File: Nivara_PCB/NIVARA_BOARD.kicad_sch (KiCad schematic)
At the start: 3 parts, among them U18 ESP32-S3-WROOM-1

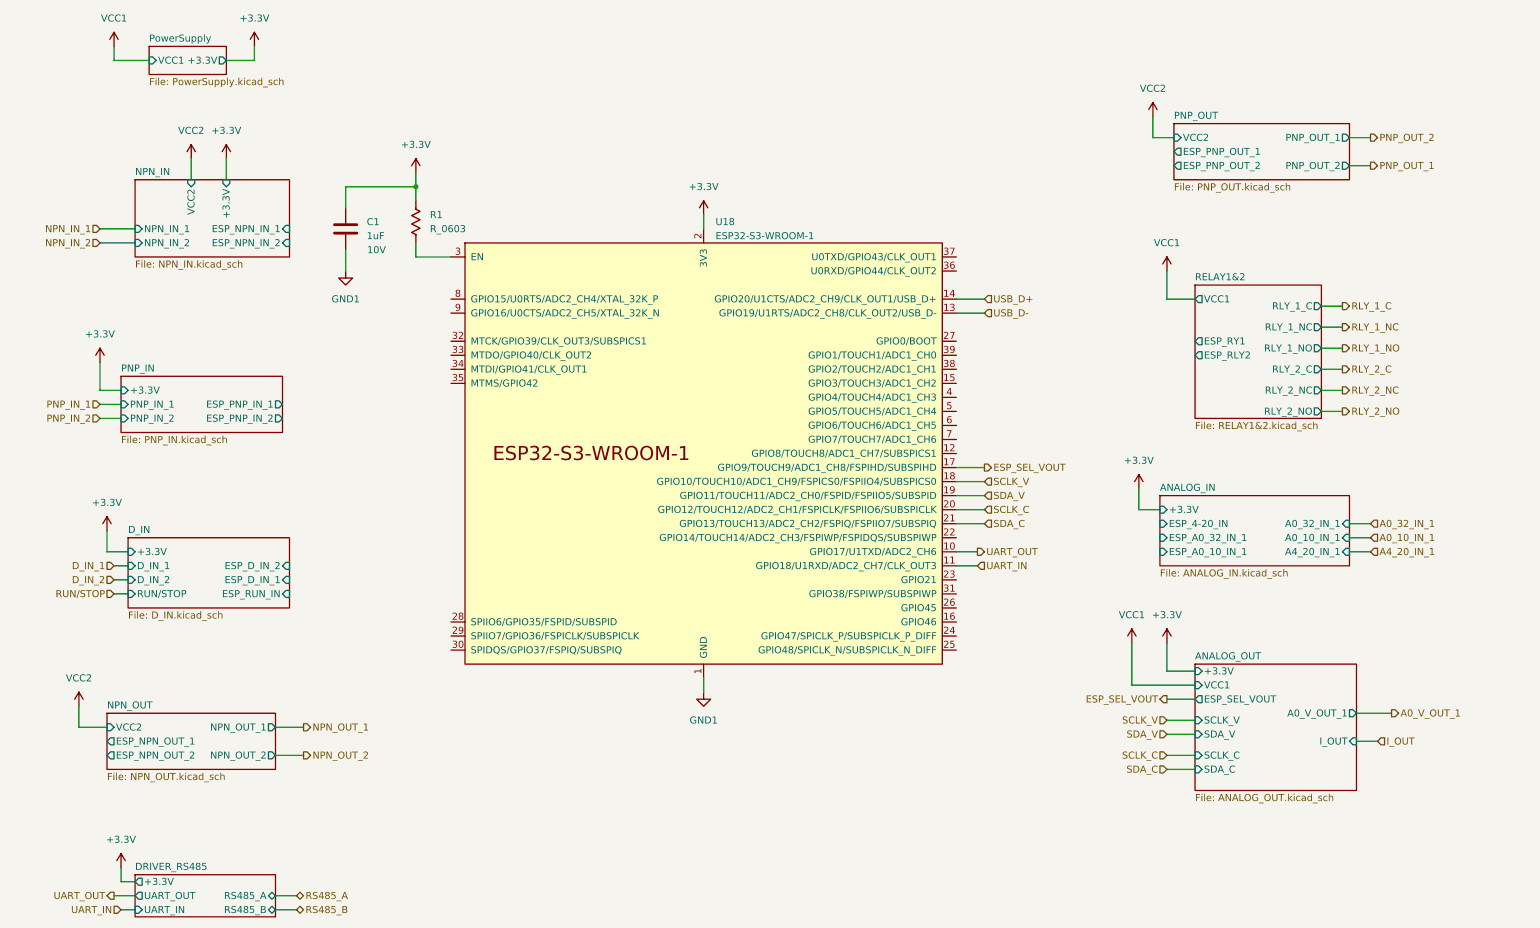
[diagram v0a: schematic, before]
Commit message: New changes to the Nivara PCB schematic files.
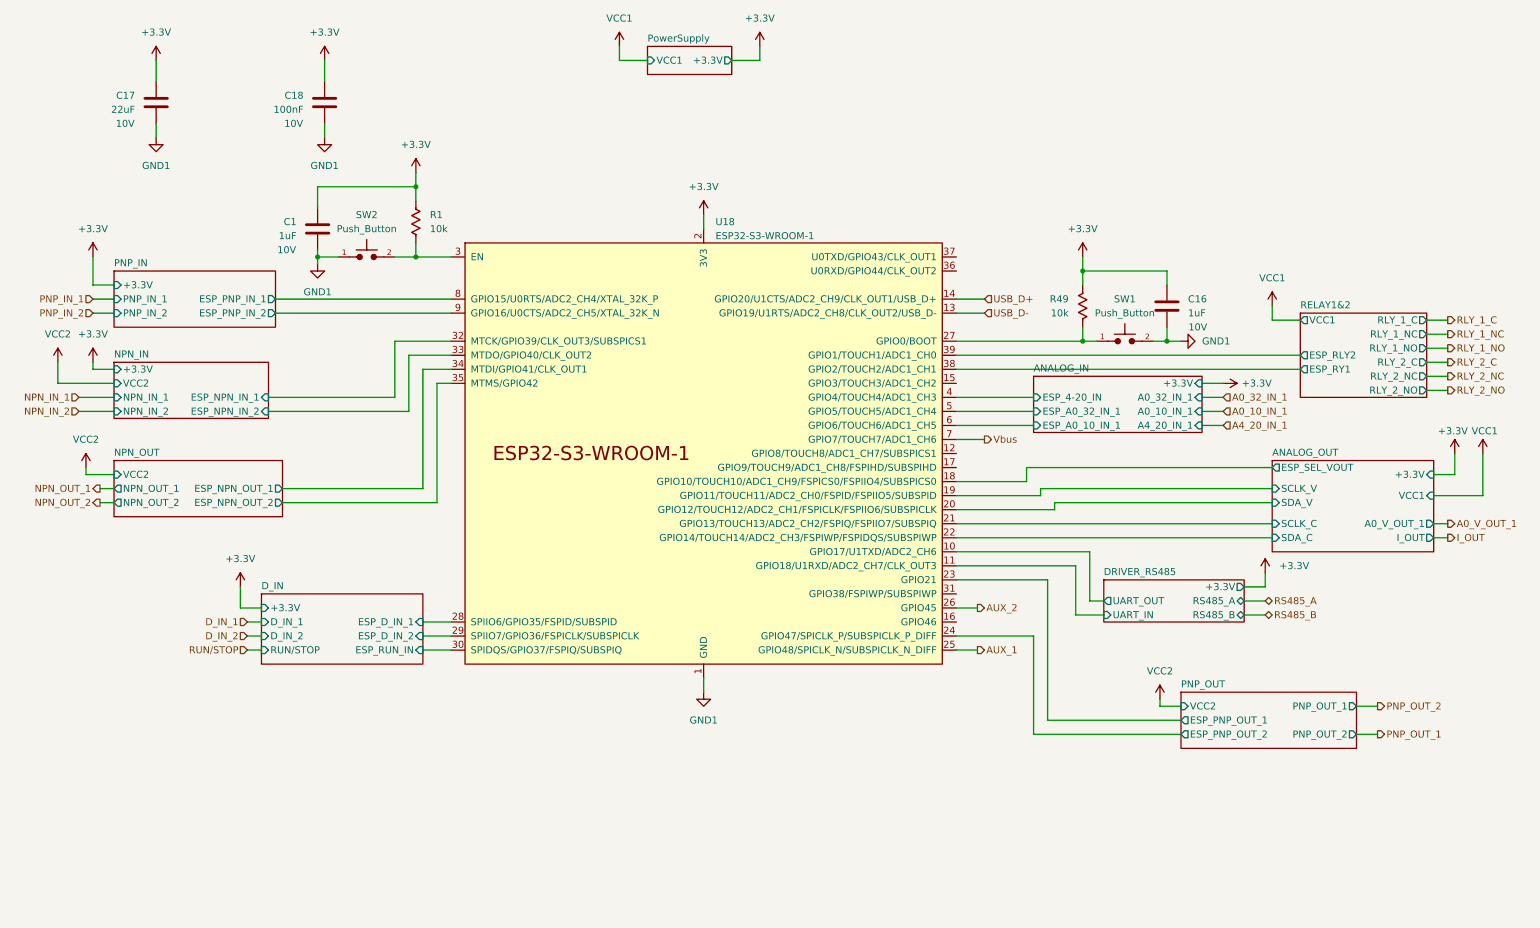
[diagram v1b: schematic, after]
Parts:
- added C16: 1uF, PCM_Capacitor_SMD_AKL:C_0603_1608Metric, symbol PCM_Capacitor_US_AKL:C_0603
- added C17: 22uF, PCM_Capacitor_SMD_AKL:C_0603_1608Metric, symbol PCM_Capacitor_US_AKL:C_0603
- added C18: 100nF, PCM_Capacitor_SMD_AKL:C_0603_1608Metric, symbol PCM_Capacitor_US_AKL:C_0603
- added R49: 10k, PCM_Resistor_SMD_AKL:R_0603_1608Metric, symbol PCM_Resistor_US_AKL:R_0603
- added SW1, SW2: Push_Button, Button_Switch_THT:SW_PUSH_6mm, symbol PCM_SL_Devices:Push_Button
- R1: value R_0603 -> 10k
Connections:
- net +3.3V: now also C16.1, C17.1, C18.1, R49.1
- net ANALOG_IN/ESP_4-20_IN: now also U18.4 (GPIO4/TOUCH4/ADC1_CH3)
- net ANALOG_IN/ESP_A0_10_IN_1: now also U18.6 (GPIO6/TOUCH6/ADC1_CH5)
- net ANALOG_IN/ESP_A0_32_IN_1: now also U18.5 (GPIO5/TOUCH5/ADC1_CH4)
- net D_IN/ESP_D_IN_1: now also U18.28 (SPIIO6/GPIO35/FSPID/SUBSPID)
- net D_IN/ESP_D_IN_2: now also U18.29 (SPIIO7/GPIO36/FSPICLK/SUBSPICLK)
- net D_IN/ESP_RUN_IN: now also U18.30 (SPIDQS/GPIO37/FSPIQ/SUBSPIQ)
- net GND1: now also C16.2, C17.2, C18.2, SW1.2, SW2.1
- net NPN_IN/ESP_NPN_IN_1: now also U18.32 (MTCK/GPIO39/CLK_OUT3/SUBSPICS1)
- net NPN_IN/ESP_NPN_IN_2: now also U18.33 (MTDO/GPIO40/CLK_OUT2)
- net NPN_OUT/ESP_NPN_OUT_1: now also U18.34 (MTDI/GPIO41/CLK_OUT1)
- net NPN_OUT/ESP_NPN_OUT_2: now also U18.35 (MTMS/GPIO42)
- net PNP_IN/ESP_PNP_IN_1: now also U18.8 (GPIO15/U0RTS/ADC2_CH4/XTAL_32K_P)
- net PNP_IN/ESP_PNP_IN_2: now also U18.9 (GPIO16/U0CTS/ADC2_CH5/XTAL_32K_N)
- net PNP_OUT/ESP_PNP_OUT_1: now also U18.23 (GPIO21)
- net PNP_OUT/ESP_PNP_OUT_2: now also U18.24 (GPIO47/SPICLK_P/SUBSPICLK_P_DIFF)
- net RELAY1&2/ESP_RLY2: now also U18.39 (GPIO1/TOUCH1/ADC1_CH0)
- net RELAY1&2/ESP_RY1: now also U18.38 (GPIO2/TOUCH2/ADC1_CH1)
- net ANALOG_OUT/SDA_C: now reaches U18.22 (GPIO14/TOUCH14/ADC2_CH3/FSPIWP/FSPIDQS/SUBSPIWP)
- net AUX_1: now reaches U18.25 (GPIO48/SPICLK_N/SUBSPICLK_N_DIFF)
- net AUX_2: now reaches U18.26 (GPIO45)
- net at U18.27 (GPIO0/BOOT): now also R49.2, SW1.1
- net at R1.2, U18.3 (EN): now also SW2.2
- net Vbus: now reaches U18.7 (GPIO7/TOUCH7/ADC1_CH6)
- net ESP_SEL_VOUT: no longer names the net of U18.17 (GPIO9/TOUCH9/ADC1_CH8/FSPIHD/SUBSPIHD)
- net SCLK_C renamed ANALOG_OUT/SDA_V
- net SCLK_V renamed ANALOG_OUT/ESP_SEL_VOUT
- net SDA_C renamed ANALOG_OUT/SCLK_C
- net SDA_V renamed ANALOG_OUT/SCLK_V
- net UART_IN renamed DRIVER_RS485/UART_IN
- net UART_OUT renamed DRIVER_RS485/UART_OUT
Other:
- moved on the sheet: C1
